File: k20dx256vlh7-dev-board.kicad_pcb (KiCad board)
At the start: 2 copper layers, 25.4 x 48.3 mm, 37 parts, among them J1 Conn_01x19_Male, J2 Conn_01x19_Male, J3 Conn_01x08_Male, J5 USB_C_Receptacle_USB2.0, SW1 Program, SW2 Reset, U1 MCP2562-E-SN, U2 MK20DX256VLH7, U4 MKL04Z32VLC4, U5 MIC5219-3.3YM5, Y1 16MHz

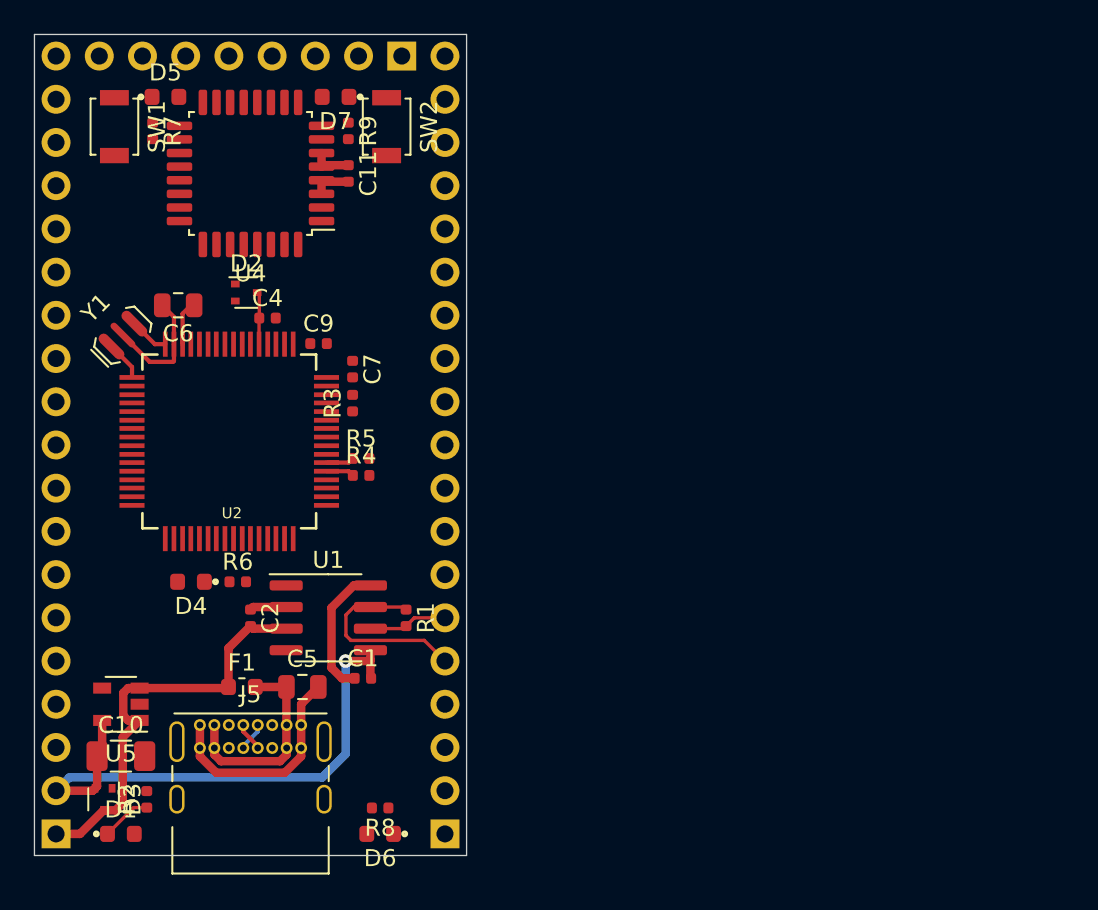
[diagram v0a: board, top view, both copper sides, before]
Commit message: 発注した！
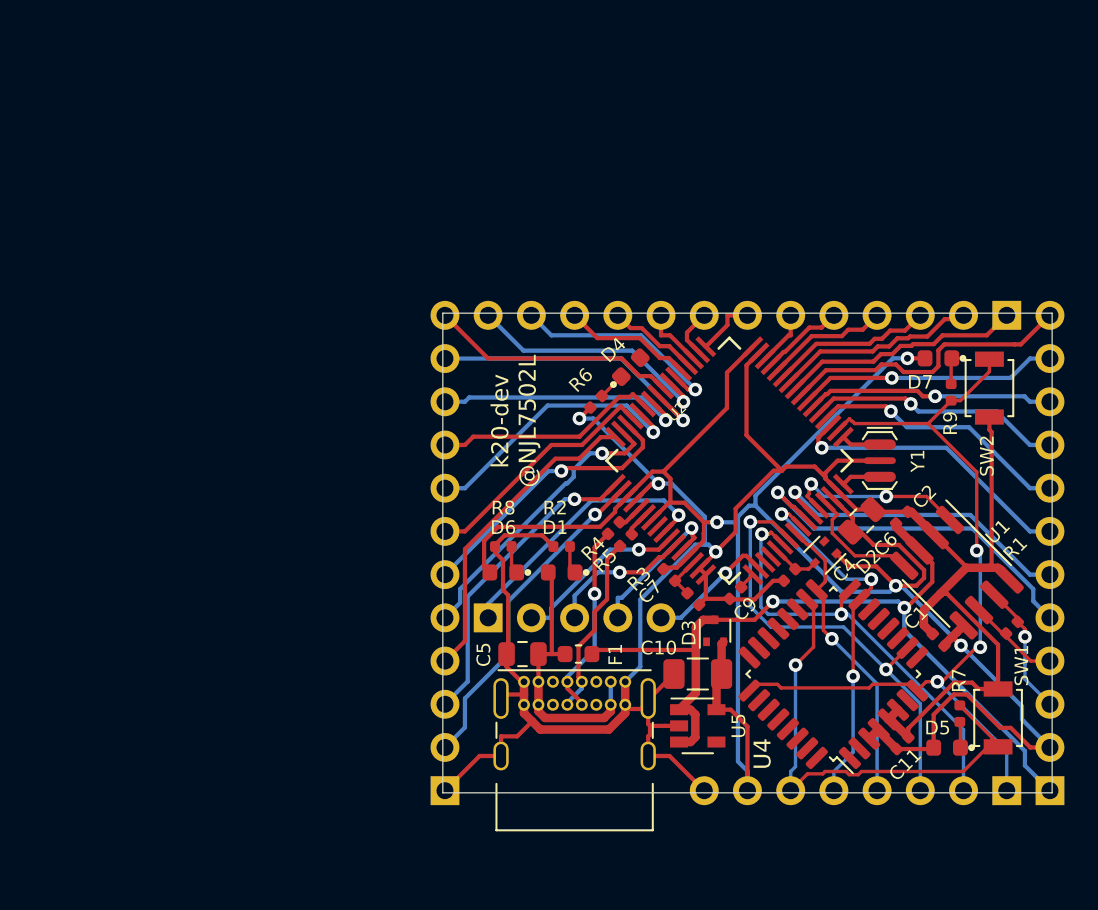
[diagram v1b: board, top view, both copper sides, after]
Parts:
- added J4: Conn_01x05_Male, Connector_PinHeader_2.54mm:PinHeader_1x05_P2.54mm_Vertical, B.Cu at (231.1, 109.2)
- added J6: Conn_01x12_Male, Connector_PinHeader_2.54mm:PinHeader_1x12_P2.54mm_Vertical, B.Cu at (264.2, 119.4)
- J1: value Conn_01x19_Male -> Conn_01x12_Male; footprint Connector_PinHeader_2.54mm:PinHeader_1x19_P2.54mm_Vertical -> Connector_PinHeader_2.54mm:PinHeader_1x12_P2.54mm_Vertical
- J2: value Conn_01x19_Male -> Conn_01x13_Male; footprint Connector_PinHeader_2.54mm:PinHeader_1x19_P2.54mm_Vertical -> Connector_PinHeader_2.54mm:PinHeader_1x13_P2.54mm_Vertical
- moved J2 63.7 mm to (261.6, 91.4), turned to 90 degrees
- moved SW1 62.5 mm to (261.1, 115.1), turned to 90 degrees
- moved D5 59.8 mm to (258.1, 116.9), turned to 180 degrees
- moved R7 58.5 mm to (258.9, 114.9), turned to 90 degrees
- moved J3 55.9 mm to (261.6, 119.4)
- moved C11 46.7 mm to (255.5, 116.6), turned to 225 degrees
- moved U4 45.2 mm to (251.4, 112.5), turned to 135 degrees
- moved Y1 45.1 mm to (254.2, 100.0), turned to 90 degrees
- moved C6 42.1 mm to (253.1, 103.5), turned to 45 degrees
- moved C2 38.7 mm to (255.5, 103.3), turned to 225 degrees
- moved D7 38.6 mm to (257.6, 94.0)
- moved R9 38.6 mm to (258.4, 96.0)
- moved SW2 38.6 mm to (260.6, 95.7)
- moved D3 37.3 mm to (244.5, 110.0), turned to 90 degrees
- moved D2 37.2 mm to (250.8, 105.5), turned to 225 degrees
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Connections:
- net Net-(J1-Pad9) renamed /D7(59)
- J1 pad 10: Net-(J1-Pad10) -> /D14(58)
- J1 pad 11: Net-(J1-Pad11) -> /D2(57)
- J1 pad 12: Net-(J1-Pad12) -> /D30(56)
- J1 pad 2: Net-(J1-Pad2) -> /D26(2)
- J1 pad 3: Net-(J1-Pad3) -> /D31(1)
- J1 pad 4: Net-(J1-Pad4) -> /D5(64)
- J1 pad 5: /CAN+ -> /D21(63)
- J1 pad 6: /CAN- -> /D20(62)
- J1 pad 7: Net-(J1-Pad7) -> /D6(61)
- J1 pad 8: Net-(J1-Pad8) -> /D8(60)
- J2 pad 1: +5V -> /D32(41)
- J2 pad 10: Net-(J2-Pad10) -> /D12(52)
- J2 pad 11: Net-(J2-Pad11) -> /D28(53)
- J2 pad 12: Net-(J2-Pad12) -> /D27(54)
- J2 pad 13: Net-(J2-Pad13) -> /D29(55)
- J2 pad 2: +3V3 -> /D25(42)
- J2 pad 3: Net-(J2-Pad3) -> /D15(43)
- J2 pad 4: Net-(J2-Pad4) -> /D22(44)
- J2 pad 5: Net-(J2-Pad5) -> /D23(45)
- J2 pad 6: Net-(J2-Pad6) -> /D9(46)
- J2 pad 7: Net-(J2-Pad7) -> /D10(49)
- J2 pad 8: Net-(J2-Pad8) -> /D13(50)_LED
- J2 pad 9: Net-(J2-Pad9) -> /D11(51)
- U2 pad 1: Net-(J2-Pad6) -> /D31(1)
- U2 pad 18: Net-(J2-Pad3) -> Net-(J4-Pad5)
- U2 pad 2: Net-(J2-Pad11) -> /D26(2)
- U2 pad 26: Net-(J2-Pad4) -> /D33(26)
- U2 pad 27: Net-(J2-Pad13) -> /D24(27)
- U2 pad 35: Net-(J1-Pad18) -> /D16(35)
- U2 pad 36: Net-(J1-Pad19) -> /D17(36)
- U2 pad 37: Net-(J2-Pad18) -> /D19(37)
- U2 pad 38: Net-(J2-Pad19) -> /D18(38)
- U2 pad 39: Net-(J1-Pad2) -> /D0(39)
- U2 pad 40: Net-(J1-Pad3) -> /D1(40)
- U2 pad 41: Net-(J2-Pad5) -> /D32(41)
- U2 pad 42: Net-(J2-Pad12) -> /D25(42)
- U2 pad 43: Net-(J1-Pad17) -> /D15(43)
- U2 pad 44: Net-(J2-Pad15) -> /D22(44)
- U2 pad 45: Net-(J2-Pad14) -> /D23(45)
- U2 pad 46: Net-(J1-Pad11) -> /D9(46)
- U2 pad 49: Net-(J1-Pad12) -> /D10(49)
- U2 pad 50: /INTERNAL_LED -> /D13(50)_LED
- U2 pad 51: Net-(J1-Pad13) -> /D11(51)
- U2 pad 52: Net-(J1-Pad14) -> /D12(52)
- U2 pad 53: Net-(J2-Pad9) -> /D28(53)
- U2 pad 54: Net-(J2-Pad10) -> /D27(54)
- U2 pad 55: Net-(J2-Pad8) -> /D29(55)
- U2 pad 56: Net-(J2-Pad7) -> /D30(56)
- U2 pad 57: Net-(J1-Pad4) -> /D2(57)
- U2 pad 58: Net-(J1-Pad16) -> /D14(58)
- U2 pad 60: Net-(J1-Pad10) -> /D8(60)
- U2 pad 61: Net-(J1-Pad8) -> /D6(61)
- U2 pad 62: Net-(J2-Pad17) -> /D20(62)
- U2 pad 63: Net-(J2-Pad16) -> /D21(63)
- U2 pad 64: Net-(J1-Pad7) -> /D5(64)
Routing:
- net GND: track 32.9 -> 144.7 mm, vias 0 -> 3
- net +3V3: track 38.1 -> 134.7 mm, vias 1 -> 4
- net /RESET: track 0.00 -> 49.0 mm, vias 0 -> 3
- net /Program: track 0.00 -> 28.6 mm, vias 0 -> 1
- net /PTA1: track 0.00 -> 26.9 mm, vias 0 -> 2
- net /PTA0: track 0.00 -> 26.0 mm, vias 0 -> 2
- net +5V: track 25.3 -> 48.7 mm, vias 0 -> 2
- net /PTA3: track 0.00 -> 21.6 mm, vias 0 -> 3
- net /D33(26): track 0.00 -> 21.6 mm, vias 0 -> 1
- net /D26(2): track 0.00 -> 19.5 mm, vias 0 -> 1
- net /D24(27): track 0.00 -> 18.7 mm, vias 0 -> 1
- net /D5(64): track 0.00 -> 18.6 mm
- net /D31(1): track 0.00 -> 18.3 mm, vias 0 -> 1
- net /PTA2: track 0.00 -> 17.7 mm, vias 0 -> 1
- net /D2(57): track 0.00 -> 17.6 mm, vias 0 -> 1
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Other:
- board size 25.4 x 48.3 mm -> 35.8 x 28.2 mm
- board text added: "k20-dev @NJL7502L"
